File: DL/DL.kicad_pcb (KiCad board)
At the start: 2 copper layers, 78 x 148.1 mm, 39 parts, among them IC1 MCP6V96UT-E_OT, IC2 SCD42-D-R2, IC3 TGS3870-B00, J3 SD_Card, J4 Conn_01x05_Male, J5 Conn_01x05_Male, J6 Conn_01x05_Male, J7 Conn_01x05_Male, Q1 BSS84, Q2 2N7002, U1 SHT31-DIS, U2 TGS5141-P00, U3 Pico

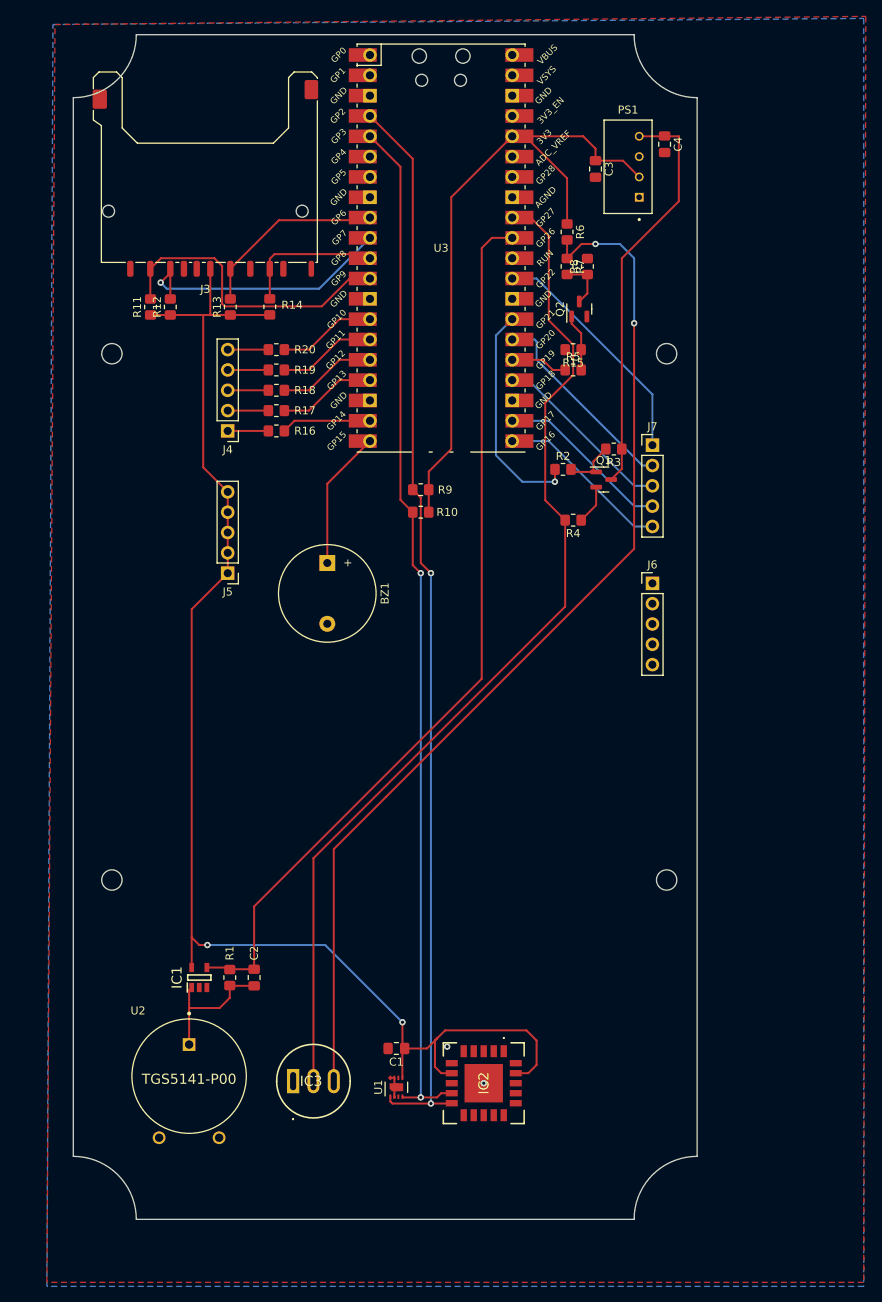
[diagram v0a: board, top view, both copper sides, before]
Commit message: Git cynchro fixed
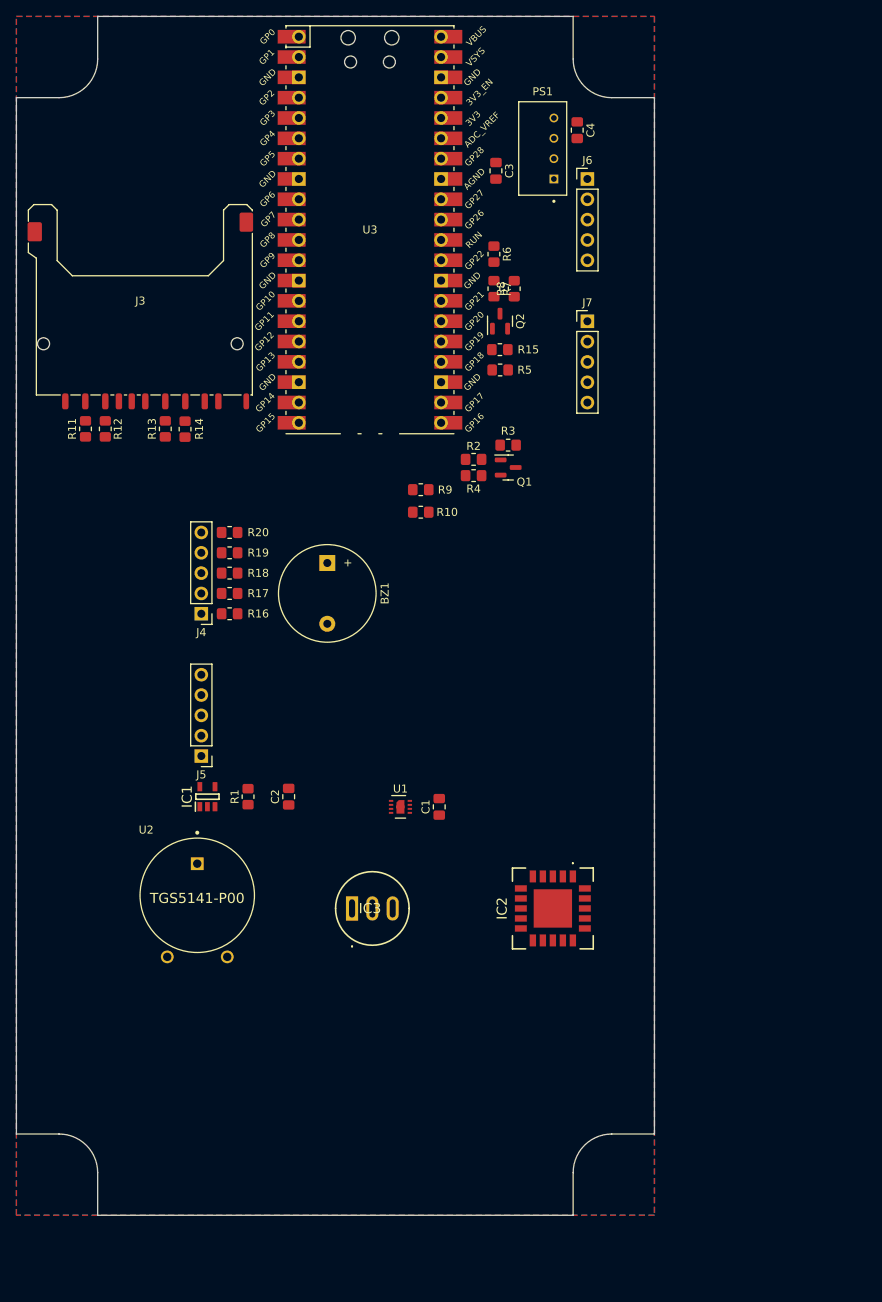
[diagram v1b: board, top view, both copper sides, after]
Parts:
- moved J6 51.2 mm to (86.9, 35.8)
- moved U1 35.1 mm to (63.5, 114.3), turned to 0 degrees
- moved C1 30.7 mm to (68.3, 114.3), turned to 90 degrees
- moved R16 23.6 mm to (42.1, 90.2)
- moved R17 23.6 mm to (42.1, 87.6)
- moved R19 23.6 mm to (42.1, 82.5)
- moved R18 23.6 mm to (42.1, 85.1)
- moved R20 23.6 mm to (42.1, 80.0)
- moved IC2 23.5 mm to (82.5, 127.0)
- moved J4 23.1 mm to (38.6, 90.2)
- moved J5 23.1 mm to (38.6, 107.9)
- moved C2 23.0 mm to (49.5, 113.0)
- moved IC3 22.8 mm to (57.5, 127.0)
- moved R1 22.7 mm to (44.5, 113.0)
- moved U2 22.6 mm to (38.1, 125.7)
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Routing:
- net +3.3V: track 258.4 -> 0.00 mm, vias 2 -> 0
- net GP2/SPI_SCK0/SDA1: track 135.0 -> 0.00 mm, vias 2 -> 0
- net VD: track 130.6 -> 0.00 mm, vias 2 -> 0
- net GP3/SPI_TX0/I2C_SCL1: track 129.3 -> 0.00 mm, vias 2 -> 0
- net GP27/ADC1/I2C_SCL1: track 128.0 -> 0.00 mm
- net GP26/ADC0/I2C_SDA1: track 112.3 -> 0.00 mm
- net +5V: track 51.4 -> 0.00 mm
- net GP9/SPI_CSn1/I2C_SCL0/UART_RX1: track 38.5 -> 0.00 mm
- net GP7/SPI_TX0/I2C_SCL1: track 35.1 -> 0.00 mm, vias 1 -> 0
- net GP22: track 29.9 -> 0.00 mm
- net GP21/I2C_SCL0: track 28.2 -> 0.00 mm, vias 1 -> 0
- net GP20/I2C_SDA0: track 25.4 -> 0.00 mm
- net GP6/SPI_SCK0/I2C_SDA1: track 23.9 -> 0.00 mm
- net GP18/SPI_SCK0/I2C_SDA1: track 23.0 -> 0.00 mm
- net GP16/SPI_RX0/I2C_SDA0/UART_TX0: track 22.0 -> 0.00 mm
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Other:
- board size 78 x 148.1 mm -> 79.8 x 149.9 mm
